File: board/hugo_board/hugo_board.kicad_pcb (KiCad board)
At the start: 2 copper layers, 49.8 x 40.1 mm, 24 parts, among them J1 Screw_Terminal_01x02, J10 Screw_Terminal_01x02, J2 Screw_Terminal_01x02, J3 Screw_Terminal_01x02, J4 Screw_Terminal_01x02, J5 Screw_Terminal_01x02, J6 Screw_Terminal_01x02, J7 Screw_Terminal_01x02, J8 Screw_Terminal_01x02, J9 Screw_Terminal_01x02, SW1 SW_Push, SW2 SW_Push, SW3 SW_Push

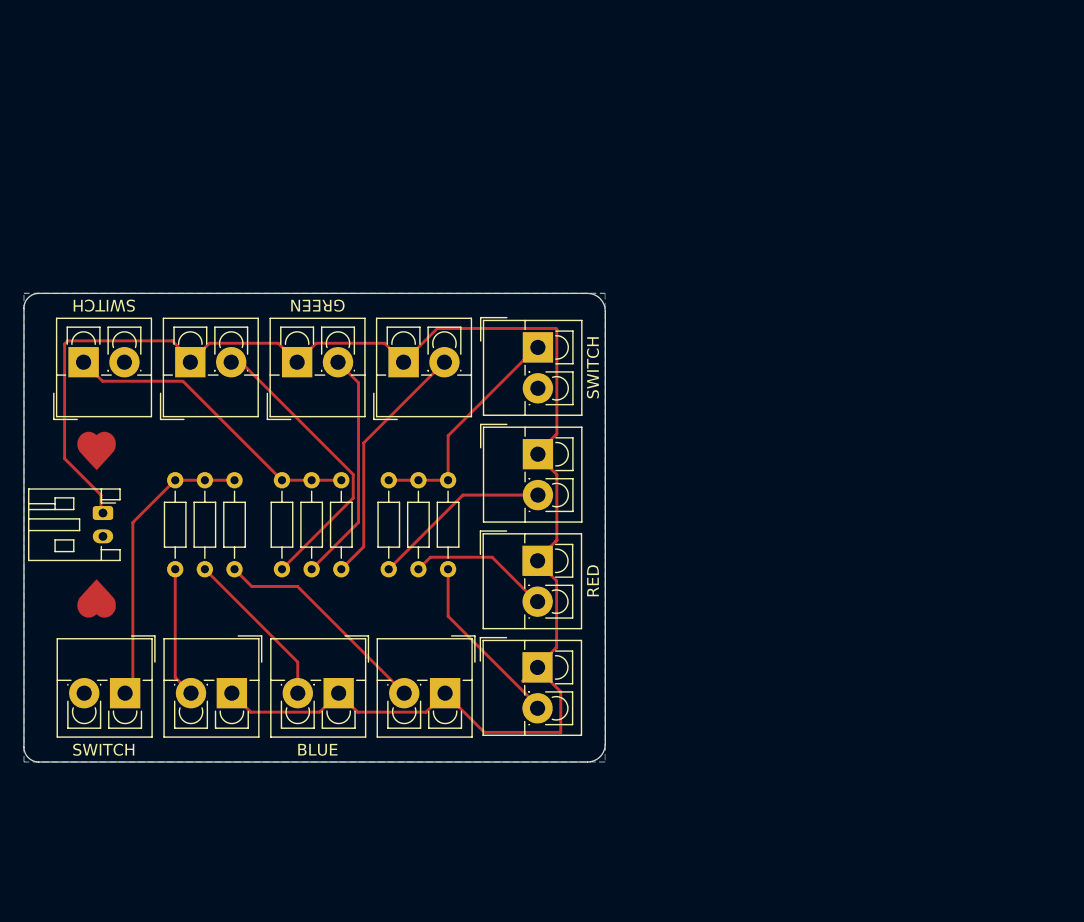
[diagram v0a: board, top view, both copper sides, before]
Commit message: version 2
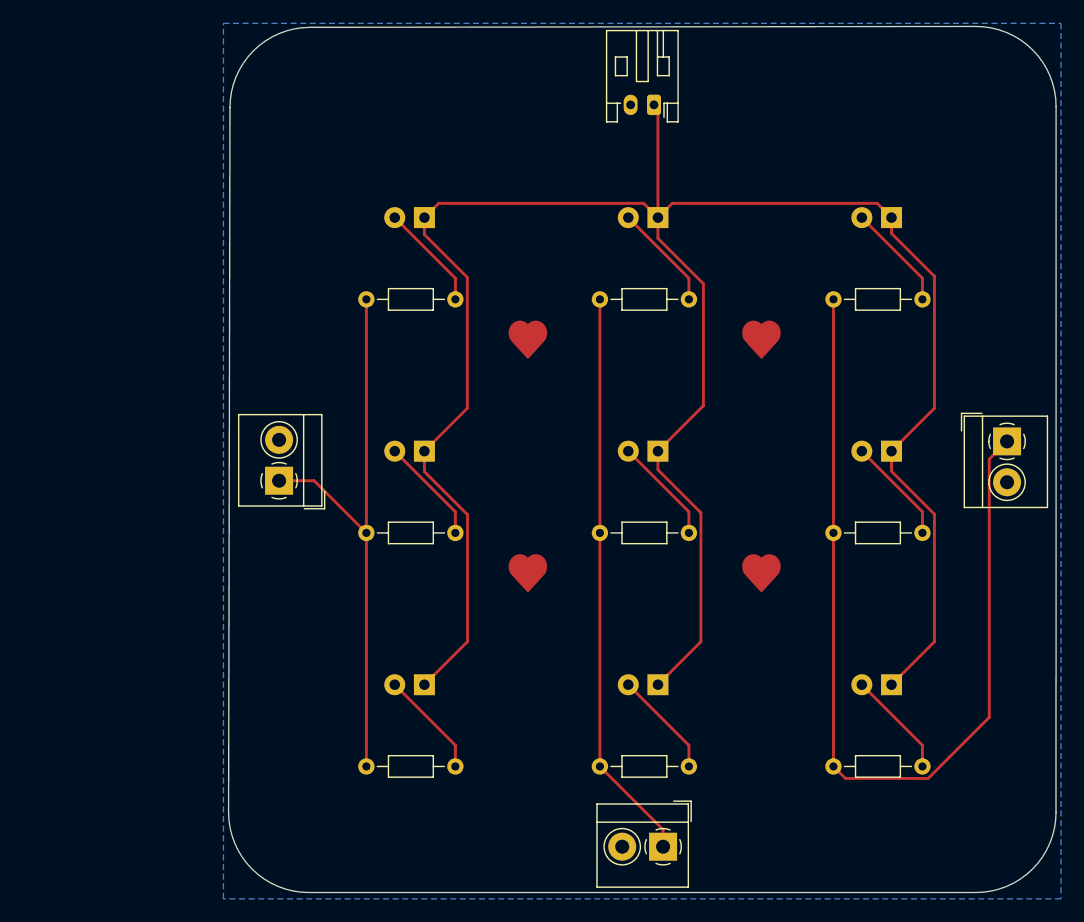
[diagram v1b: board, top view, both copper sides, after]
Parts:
- removed the J1 at (117.1, 105.6)
- removed J10, J2, J3, J4, J5, J6, J8, J9: Screw_Terminal_01x02, TerminalBlock_4Ucon:TerminalBlock_4Ucon_1x02_P3.50mm_Vertical
- removed the Ref** at (105.7, 97.5)
- removed the Ref** at (105.4, 84.8)
- removed the SW1 at (108.0, 105.6)
- added BLUE1: LED, LED_THT:LED_D10.0mm, B.Cu at (133.6, 64.9)
- added BLUE2: LED, LED_THT:LED_D10.0mm, B.Cu at (133.6, 84.9)
- added BLUE3: LED, LED_THT:LED_D10.0mm, B.Cu at (133.6, 104.9)
- added GREEN1: LED, LED_THT:LED_D10.0mm, B.Cu at (153.6, 64.9)
- added GREEN2: LED, LED_THT:LED_D10.0mm, B.Cu at (153.6, 84.9)
- added GREEN3: LED, LED_THT:LED_D10.0mm, B.Cu at (153.6, 104.9)
- added RED1: LED, LED_THT:LED_D10.0mm, B.Cu at (173.6, 64.9)
- added RED2: LED, LED_THT:LED_D10.0mm, B.Cu at (173.6, 84.9)
- added RED3: LED, LED_THT:LED_D10.0mm, B.Cu at (173.6, 104.9)
- added Ref**: Val**, art:drawing, F.Cu at (142.3, 95.3)
- added Ref**: Val**, art:drawing, F.Cu at (162.3, 95.3)
- added Ref**: Val**, art:drawing, F.Cu at (142.3, 75.3)
- added Ref**: Val**, art:drawing, F.Cu at (162.3, 75.3)
- added SW3: SW_Push, TerminalBlock_4Ucon:TerminalBlock_4Ucon_1x02_P3.50mm_Horizontal, F.Cu at (154.1, 118.8)
- SW1: renamed from SW3; footprint TerminalBlock_4Ucon:TerminalBlock_4Ucon_1x02_P3.50mm_Vertical -> TerminalBlock_4Ucon:TerminalBlock_4Ucon_1x02_P3.50mm_Horizontal
- SW2: footprint TerminalBlock_4Ucon:TerminalBlock_4Ucon_1x02_P3.50mm_Vertical -> TerminalBlock_4Ucon:TerminalBlock_4Ucon_1x02_P3.50mm_Horizontal
- moved J1 58.7 mm to (153.3, 55.2), turned to 180 degrees
- moved R4 51.2 mm to (176.3, 71.9), turned to 180 degrees
- moved R6 44.0 mm to (176.3, 111.9), turned to 180 degrees
- moved R5 43.3 mm to (176.3, 91.9), turned to 180 degrees
- moved R7 41.8 mm to (156.3, 71.9), turned to 180 degrees
- moved SW2 41.0 mm to (183.5, 84.0)
- moved R9 34.2 mm to (156.3, 111.9), turned to 180 degrees
- moved R1 33.3 mm to (136.3, 71.9), turned to 180 degrees
- moved R8 32.5 mm to (156.3, 91.9), turned to 180 degrees
- moved R3 25.4 mm to (136.3, 111.9), turned to 180 degrees
- moved R2 21.7 mm to (136.3, 91.9), turned to 180 degrees
- moved SW1 19.6 mm to (121.2, 87.4), turned to 90 degrees
- renumbered J7 to J1
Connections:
- SW1 pad 1: Net-(R7-Pad2) -> Net-(R1-Pad2)
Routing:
- net Net-(R4-Pad2): track 19.6 -> 80.7 mm
- net +BATT: track 136.5 -> 190.3 mm
- net Net-(R1-Pad2): track 25.1 -> 49.3 mm
- net Net-(R7-Pad2): track 26.3 -> 49.1 mm
- net Net-(GREEN1-Pad2): track 24.2 -> 9.15 mm
- net Net-(GREEN3-Pad2): track 21.4 -> 9.15 mm
- net Net-(GREEN2-Pad2): track 20.1 -> 9.15 mm
- net Net-(BLUE3-Pad2): track 18.9 -> 9.15 mm
- net Net-(R4-Pad1): track 15.3 -> 9.15 mm
- net Net-(R6-Pad1): track 15.0 -> 9.15 mm
- net Net-(BLUE2-Pad2): track 13.9 -> 9.15 mm
- net Net-(R5-Pad1): track 12.1 -> 9.15 mm
- net Net-(BLUE1-Pad2): track 11.2 -> 9.15 mm
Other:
- board size 49.8 x 40.1 mm -> 70.9 x 74.2 mm
- board text added: "V2"
- board text removed: "BLUE"
- board text removed: "GREEN"
- board text removed: "RED"
- board text removed: "SWITCH"
